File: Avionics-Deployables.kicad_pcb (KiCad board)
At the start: 2 copper layers, 82.6 x 90 mm, 0 parts

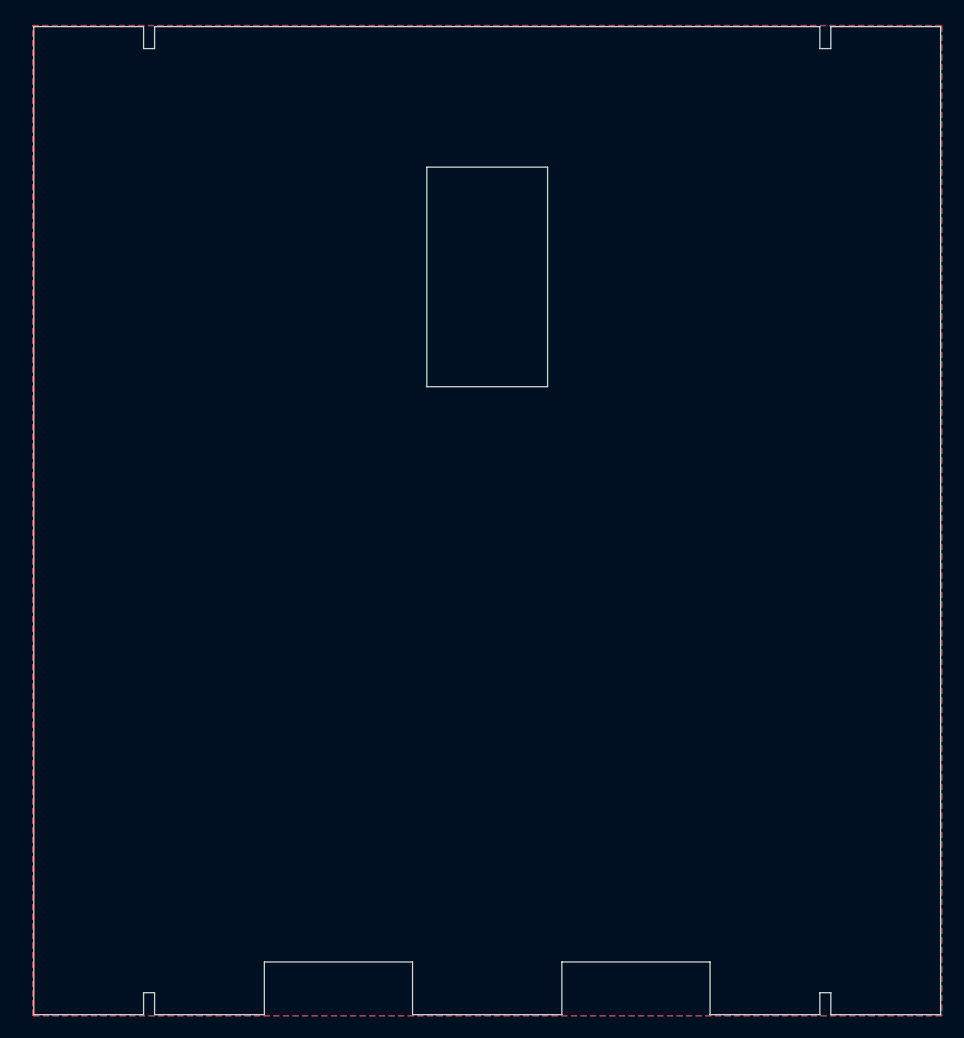
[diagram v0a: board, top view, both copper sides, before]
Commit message: Export BOM
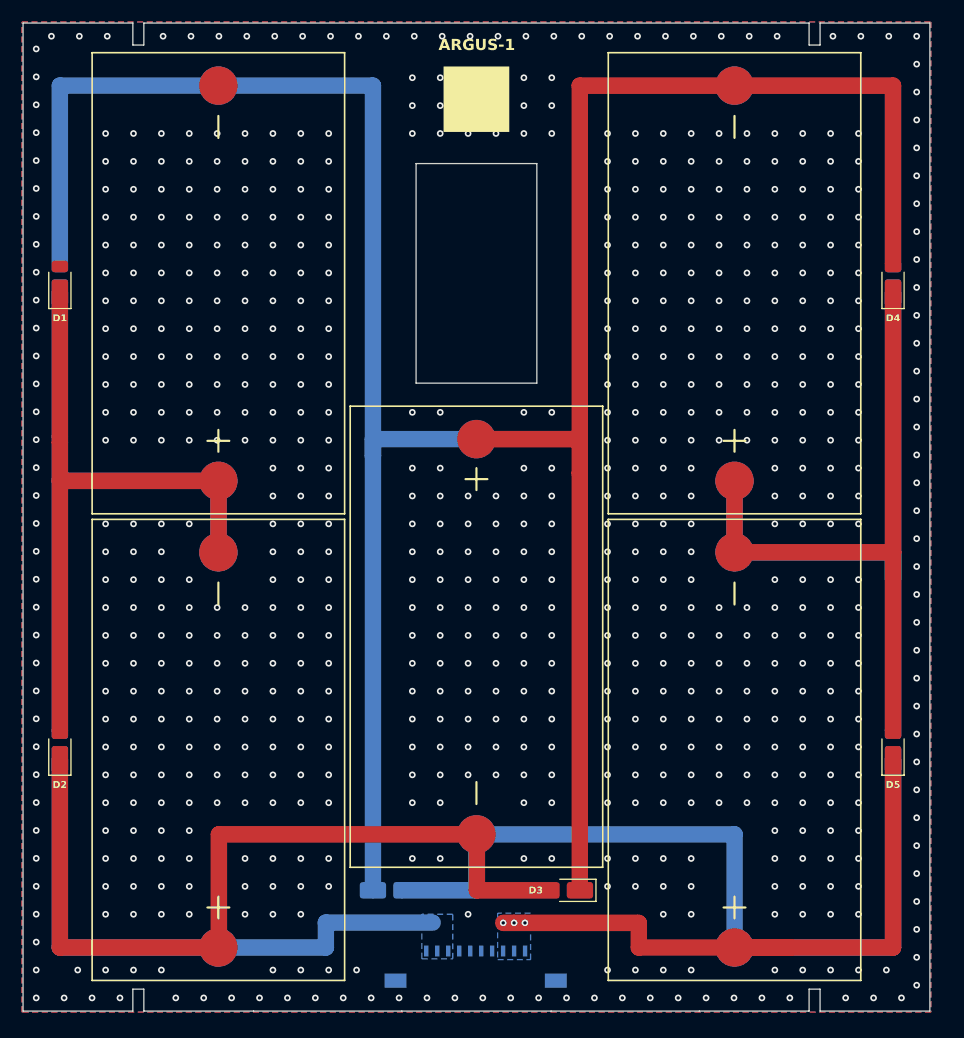
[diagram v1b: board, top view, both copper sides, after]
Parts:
- added D1: DFLS130L-7, Diode_SMD:D_PowerDI-123, F.Cu at (109.4, 74.5)
- added D10: DFLS130L-7, Diode_SMD:D_PowerDI-123, B.Cu at (109.4, 117.0)
- added D2: DFLS130L-7, Diode_SMD:D_PowerDI-123, F.Cu at (109.4, 117.0)
- added D3: DFLS130L-7, Diode_SMD:D_PowerDI-123, F.Cu at (155.9, 129.8)
- added D4: DFLS130L-7, Diode_SMD:D_PowerDI-123, F.Cu at (185.3, 74.5)
- added D5: DFLS130L-7, Diode_SMD:D_PowerDI-123, F.Cu at (185.3, 117.0)
- added D6: DFLS130L-7, Diode_SMD:D_PowerDI-123, B.Cu at (185.3, 74.5)
- added D7: DFLS130L-7, Diode_SMD:D_PowerDI-123, B.Cu at (185.3, 117.0)
- added D8: DFLS130L-7, Diode_SMD:D_PowerDI-123, B.Cu at (138.7, 129.8)
- added D9: DFLS130L-7, Diode_SMD:D_PowerDI-123, B.Cu at (109.4, 74.5)
- added J1: 200528-0100, Connector_FFC-FPC:Molex_200528-0100_1x10-1MP_P1.00mm_Horizontal, B.Cu at (147.3, 136.2)
- added SC1: SM141K06TF, SolarPanels:SM141K06TF, F.Cu at (123.8, 74.5)
- added SC10: SM141K06TF, SolarPanels:SM141K06TF, B.Cu at (123.8, 117.0)
- added SC2: SM141K06TF, SolarPanels:SM141K06TF, F.Cu at (123.8, 117.0)
- added SC3: SM141K06TF, SolarPanels:SM141K06TF, F.Cu at (147.3, 106.7)
- added SC4: SM141K06TF, SolarPanels:SM141K06TF, F.Cu at (170.8, 74.5)
- added SC5: SM141K06TF, SolarPanels:SM141K06TF, F.Cu at (170.8, 117.0)
- added SC6: SM141K06TF, SolarPanels:SM141K06TF, B.Cu at (170.8, 74.5)
- added SC7: SM141K06TF, SolarPanels:SM141K06TF, B.Cu at (170.8, 117.0)
- added SC8: SM141K06TF, SolarPanels:SM141K06TF, B.Cu at (147.3, 106.7)
- added SC9: SM141K06TF, SolarPanels:SM141K06TF, B.Cu at (123.8, 74.5)
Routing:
- net Net-(D3-K): track 0.00 -> 130.5 mm
- net Net-(D8-K): track 0.00 -> 128.9 mm
- net Net-(D7-K): track 0.00 -> 77.3 mm
- net Net-(D2-K): track 0.00 -> 77.2 mm
- net Net-(D6-K): track 0.00 -> 63.2 mm
- net Net-(D4-K): track 0.00 -> 60.8 mm
- net Net-(D1-K): track 0.00 -> 60.8 mm
- net Net-(D10-A): track 0.00 -> 60.7 mm
- net D_VSOLAR1: track 0.00 -> 59.9 mm, vias 0 -> 3
- net D_VSOLAR2: track 0.00 -> 53.4 mm
- net GND: vias 0 -> 741
- added copper zone on B.Cu, net D_VSOLAR1
- added copper zone on B.Cu, net D_VSOLAR2
- added copper zone on B.Cu, net GND
- added copper zone on F.Cu, net GND
- removed copper zone on B.Cu, net (none)
- removed copper zone on F.Cu, net (none)
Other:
- outline, holes or cut-outs redrawn
- board text added: "1"
- board text added: "10"
- board text added: "ARGUS-1"
- board text added: "DVSOLAR1"
- board text added: "DVSOLAR2"
- board text added: "GND"
- board text added: "TO X/Y SOLAR PANEL"
- board text removed: "Solar Deployables Mechanical Stand-in 0.8mm"
